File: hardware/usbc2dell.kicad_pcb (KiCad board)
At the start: 2 copper layers, 39.5 x 26.5 mm, 27 parts, among them J1 TYPE-C-31-M-17, J2 WJ15EDGRC-3.81-3P, Q1 DOD50P06, Q2 MMBT5551, SW1 DSWB04LHGET, U1 ATtiny1616-M, U2 FUSB302BMPX, U3 L7805, U4 SRV05-4

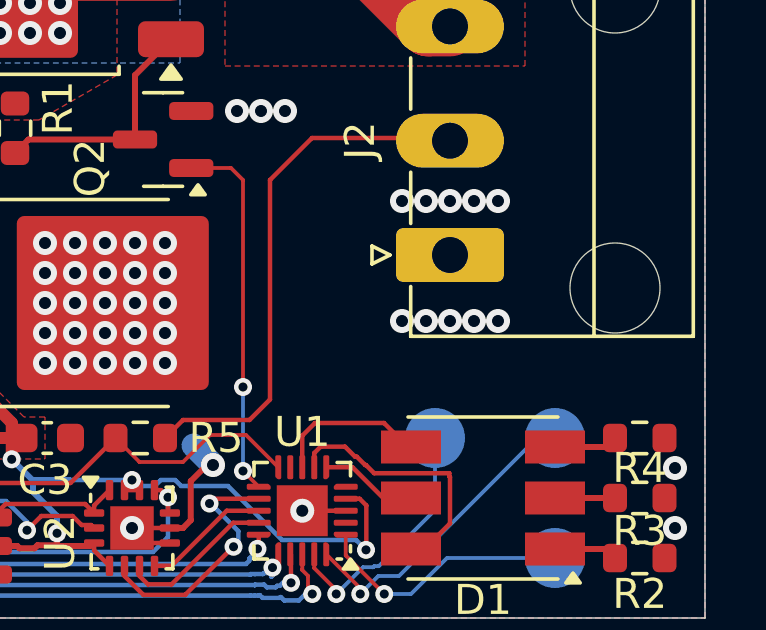
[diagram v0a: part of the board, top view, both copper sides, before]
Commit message: stuff
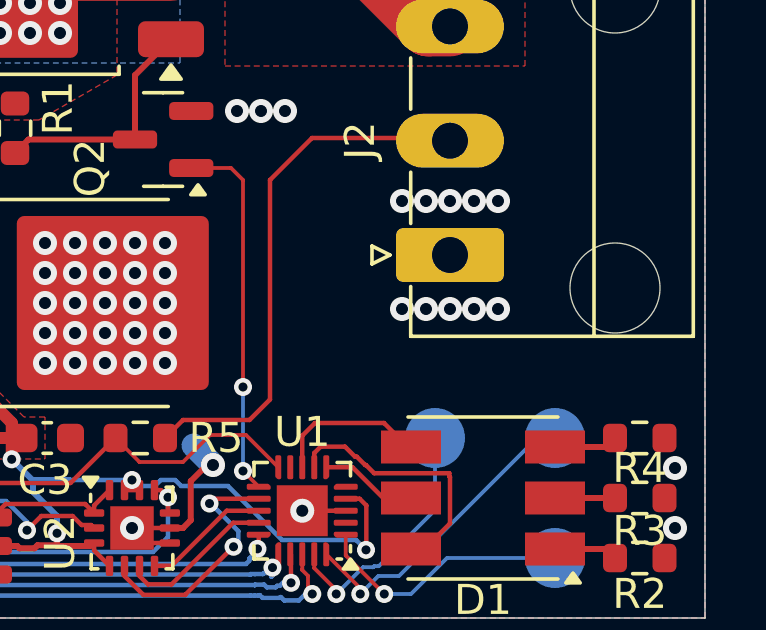
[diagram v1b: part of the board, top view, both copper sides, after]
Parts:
- moved ICON1 0.22 mm to (25.2, 42.6)
